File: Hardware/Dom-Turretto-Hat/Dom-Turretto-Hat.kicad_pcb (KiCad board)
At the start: 2 copper layers, 65 x 56 mm, 53 parts, among them J1 Raspberry_Pi_2_3, J2 Conn_01x02, J3 Barrel_Jack_Switch, Q1 SI4143DY-T1-GE3, Q2 SI4143DY-T1-GE3, U1 CAT24C32WI-GT3, U2 LM22679TJ-5.0/NOPB, U3 LTC4412xS6, U4 LTC4411ES5TRMPBF

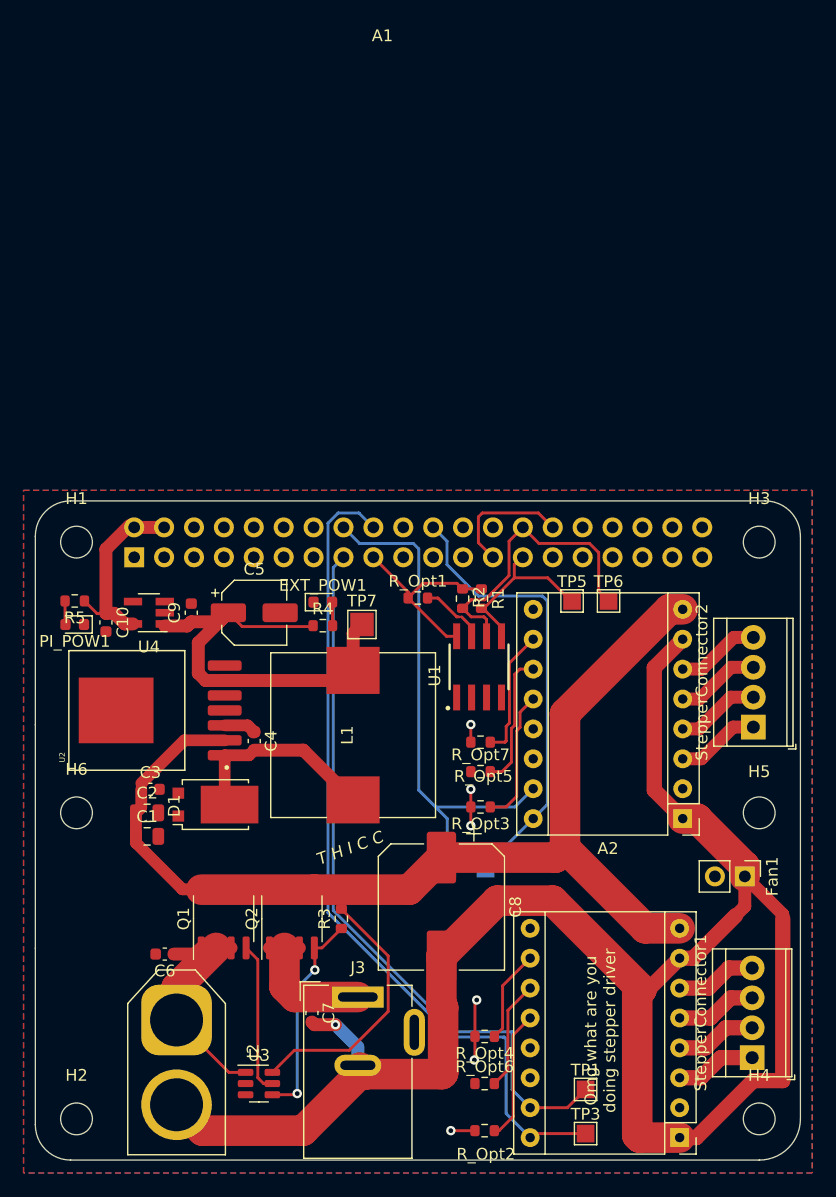
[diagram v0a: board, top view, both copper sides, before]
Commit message: Make final changes
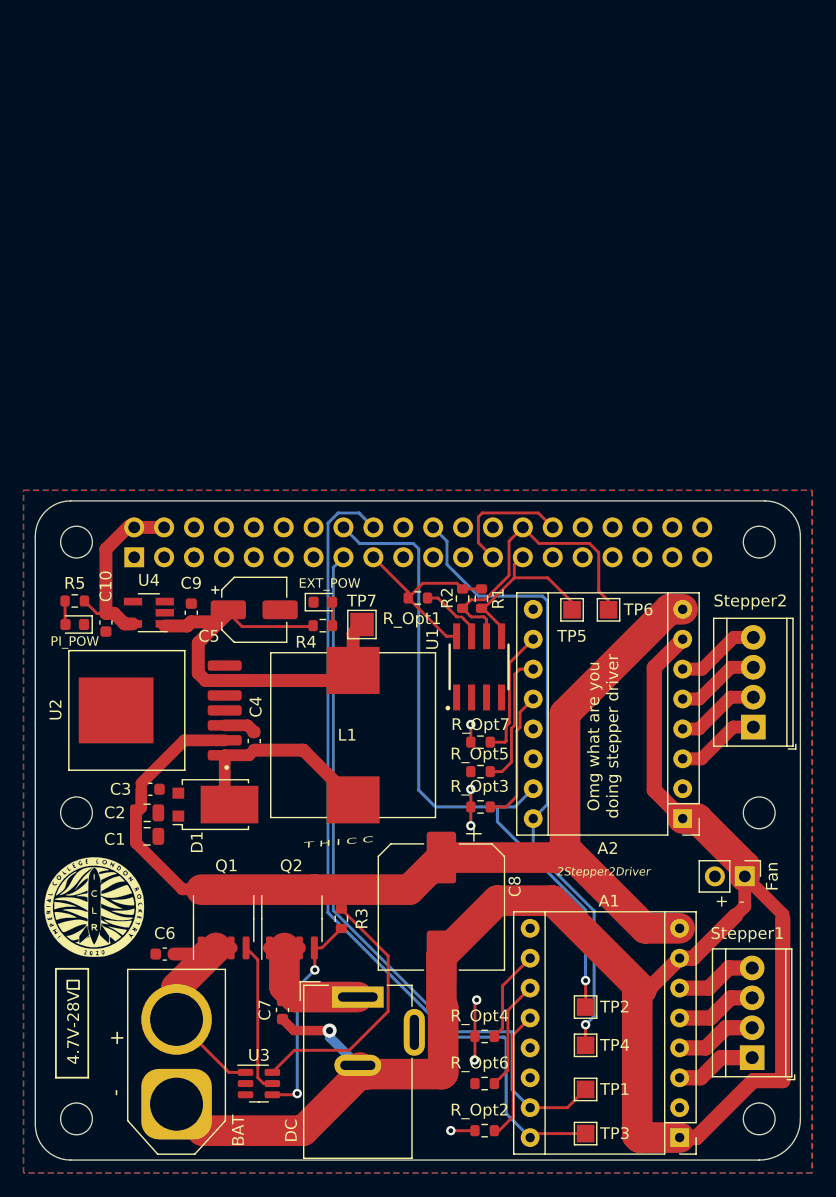
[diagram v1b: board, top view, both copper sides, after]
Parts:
- added G***: LOGO, iclr:iclr_logo, F.Cu at (116.5, 112.5)
- added G***: LOGO, iclr:Dom_License, B.Cu at (144.0, 105.0)
- TP2, TP4: moved to F.Cu
- moved TP4 17.2 mm to (158.2, 124.2), turned to 0 degrees
- moved TP2 16.6 mm to (158.2, 121.0), turned to 0 degrees
- moved BAT 7.15 mm to (123.5, 129.2), turned to 90 degrees
- moved C7 2.51 mm to (132.5, 121.2)
- moved TP5 0.75 mm to (157.1, 87.2)
- moved TP6 0.75 mm to (160.2, 87.2)
- moved C5 0.25 mm to (130.1, 87.2)
- renumbered J2 to BAT, J3 to DC, EXT_POW1 to EXT_POW, Fan1 to Fan, PI_POW1 to PI_POW, StepperConnector1 to Stepper1, StepperConnector2 to Stepper2
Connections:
- BAT pad 1: Net-(C6-Pad1) -> GND
- BAT pad 2: GND -> Net-(C6-Pad1)
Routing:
- net /Dir2: track 38.4 -> 54.1 mm, vias 0 -> 1
- net /Step2: track 44.3 -> 58.7 mm, vias 0 -> 1
- net GND: track 160.8 -> 162.8 mm
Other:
- board text added: "+ -"
- board text added: "0"
- board text added: "2Stepper2Driver"
- board text added: "4.7V-28V⎓"
- board text added: "JLCJLCJLCJLCJLCJLC"
- board text added: "Shitposted with <3 by Daniele Bella"
